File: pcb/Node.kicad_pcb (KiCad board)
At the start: 4 copper layers, 50 x 50 mm, 163 parts, among them J1 LCD, J10 SPI, J11 GPA[0..3], J13 Power In, J14 SERIAL, J2 USB_C_USB2.0_16P, J3 INDICATOR, J4 GPB[0..3], J5 GPB[4..7], J6 BTN[0..3], J7 GPA[4..7], J8 QWIIC1, J9 QWIIC2, Q1 MMBT2222A, SW1 RESET, SW2 BOOT, U1 ESP32-S3-WROOM-1-N8R2, U2 LM66200DRLR, U3 USBLC6-2P6, U4 MCP23017T-E/ML, U6 LM66200DRLR, U7 AZ1084-3.3

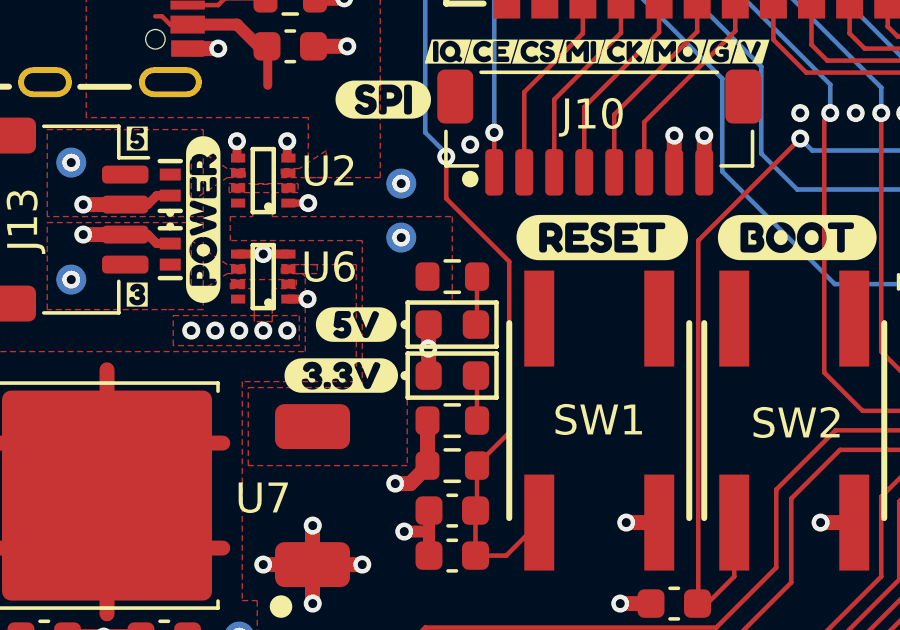
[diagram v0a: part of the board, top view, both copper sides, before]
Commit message: Continued rationalizing parts
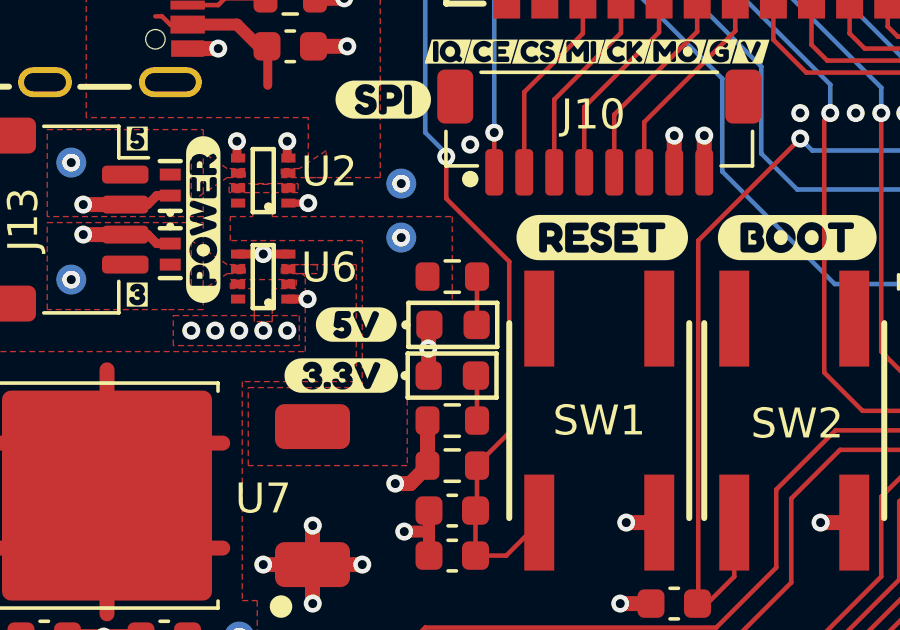
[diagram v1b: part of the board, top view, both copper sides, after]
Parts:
- D23: value Orange -> Blue
